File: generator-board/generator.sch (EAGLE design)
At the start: 42 parts, among them IC1 MAX1771, J2 HV_GEN-HOLE, Q1 IRF740DPACK

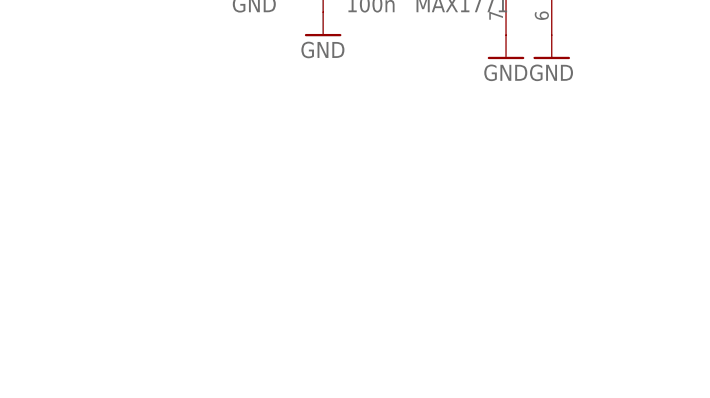
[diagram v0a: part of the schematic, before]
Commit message: about to panelize
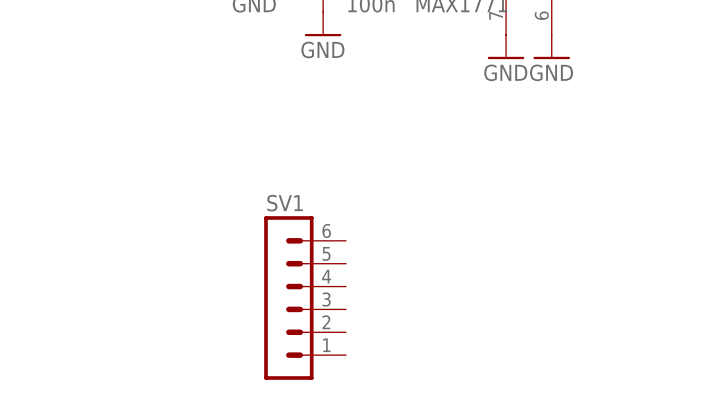
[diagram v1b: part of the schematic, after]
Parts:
- added SV1: (no value), con-lstb:MA06-1
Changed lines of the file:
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@@
 <?xml version="1.0" encoding="utf-8"?>
 <!DOCTYPE eagle SYSTEM "eagle.dtd">
-<eagle version="6.5.0">
+<eagle version="6.6.0">
 <drawing>
 <settings>
@@
 <part name="GND13" library="supply1" deviceset="GND" device=""/>
 <part name="GND14" library="supply1" deviceset="GND" device=""/>
+<part name="SV1" library="con-lstb" deviceset="MA06-1" device=""/>
 </parts>
 <sheets>
@@
 <instance part="GND13" gate="1" x="167.64" y="12.7"/>
 <instance part="GND14" gate="1" x="137.16" y="17.78"/>
+<instance part="SV1" gate="1" x="12.7" y="10.16"/>
 </instances>
 <busses>

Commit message: final board, started firmware
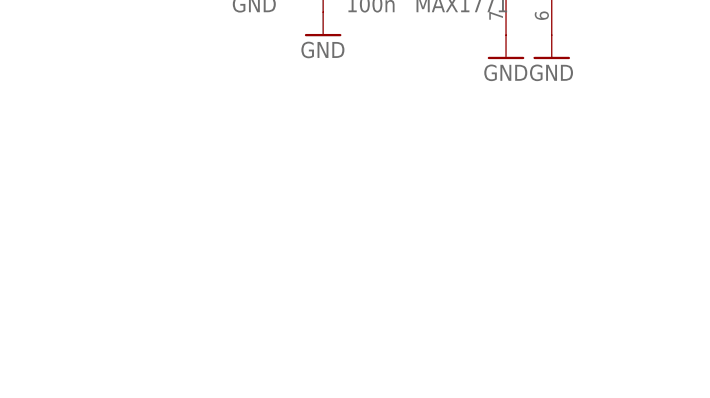
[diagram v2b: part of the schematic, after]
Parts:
- removed SV1: (no value), con-lstb:MA06-1
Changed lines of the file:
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@@
 <part name="GND13" library="supply1" deviceset="GND" device=""/>
 <part name="GND14" library="supply1" deviceset="GND" device=""/>
-<part name="SV1" library="con-lstb" deviceset="MA06-1" device=""/>
 </parts>
 <sheets>
@@
 <instance part="GND13" gate="1" x="167.64" y="12.7"/>
 <instance part="GND14" gate="1" x="137.16" y="17.78"/>
-<instance part="SV1" gate="1" x="12.7" y="10.16"/>
 </instances>
 <busses>
